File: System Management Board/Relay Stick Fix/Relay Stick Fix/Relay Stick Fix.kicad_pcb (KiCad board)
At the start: 4 copper layers, 28.2 x 27 mm, 17 parts, among them J1 Conn_02x06, Q1 NMOS, U2 74LVC1G04

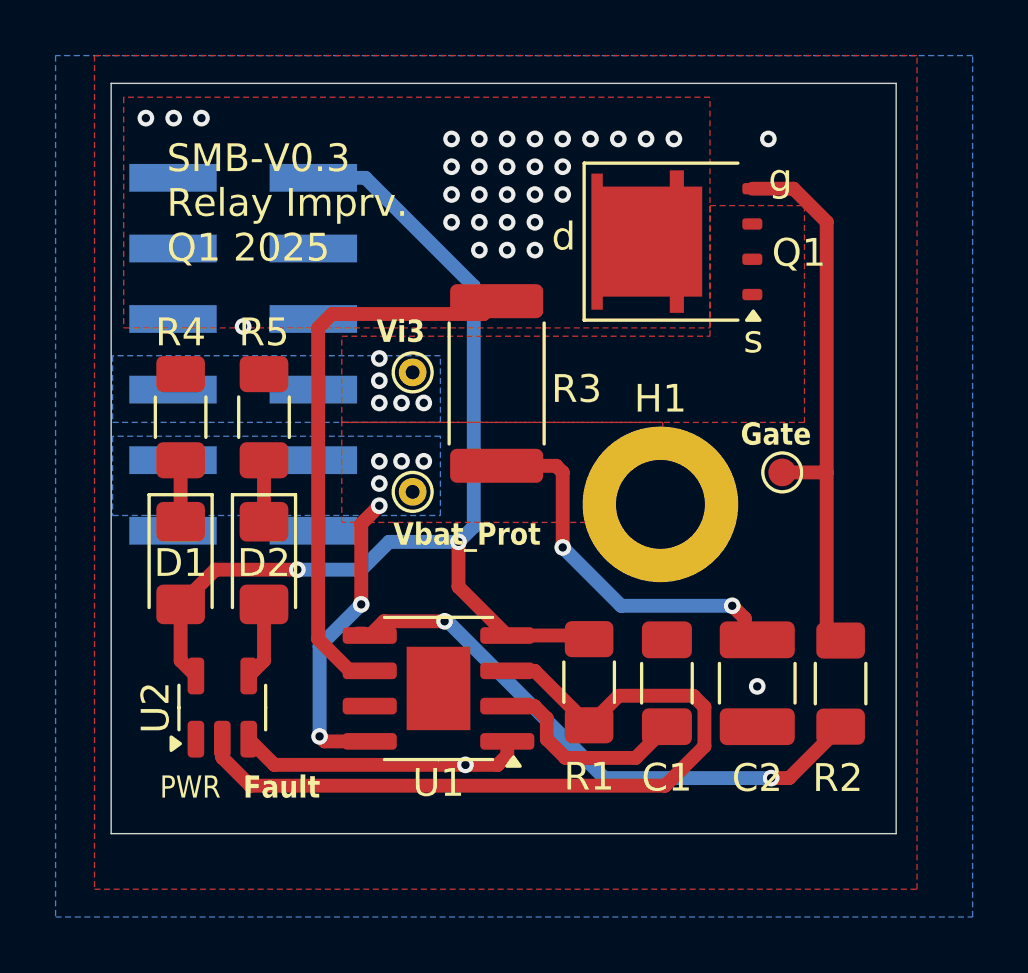
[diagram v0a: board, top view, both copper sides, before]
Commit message: zone fix
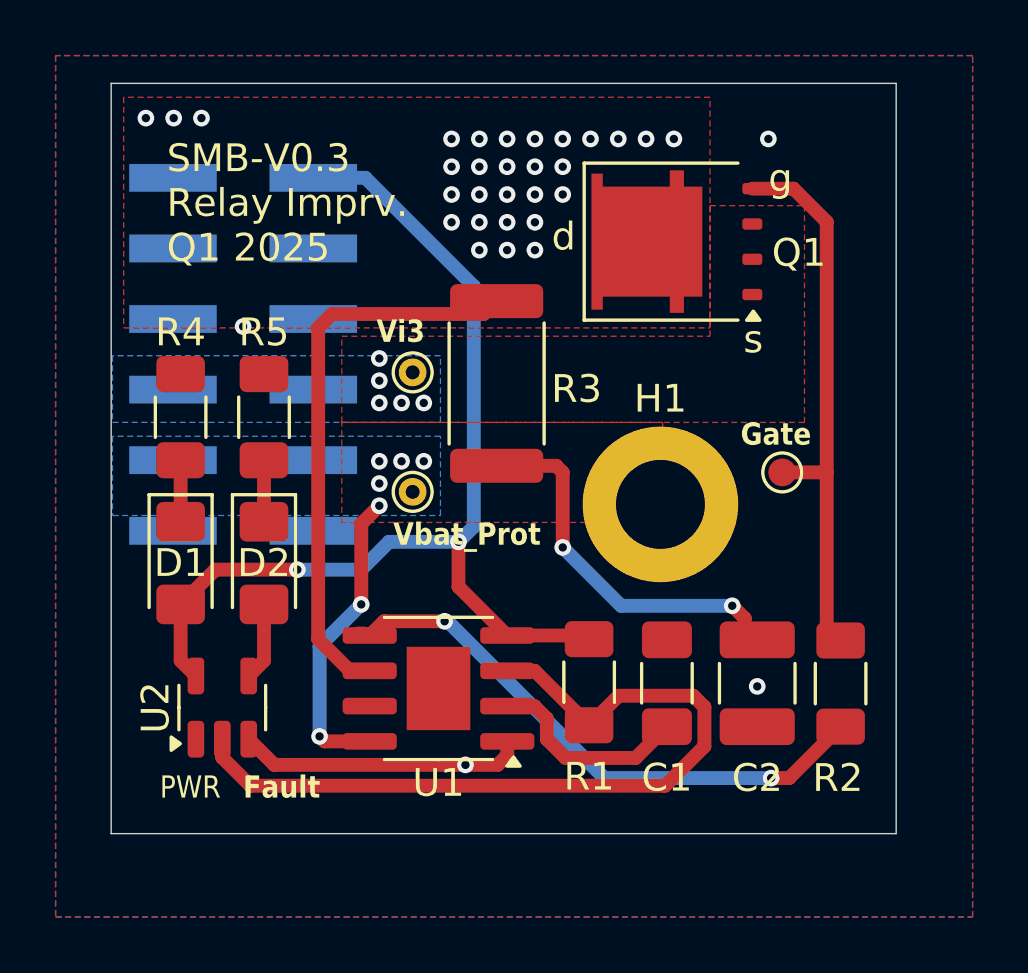
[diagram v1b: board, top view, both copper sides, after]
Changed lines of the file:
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@@
 		(net 1)
 		(net_name "GND")
-		(layers "F.Cu" "In1.Cu")
-		(hatch edge 0.5)
-		(priority 1)
-		(connect_pads
-			(clearance 0.5)
-		)
-		(min_thickness 0.25)
-		(filled_areas_thickness no)
-		(fill yes
-			(thermal_gap 0.5)
-			(thermal_bridge_width 0.5)
-		)
-		(polygon
-			(pts
-				(xy 15.25 14) (xy 15.25 44) (xy 44.85 44) (xy 44.85 14)
-			)
-		)
-	)
-	(zone
-		(net 1)
-		(net_name "GND")
-		(layers "In1.Cu" "B.Cu")
+		(layers "F.Cu" "In1.Cu" "B.Cu")
 		(hatch edge 0.5)
 		(connect_pads
@@
 			)
 		)
+	)
+	(zone
+		(net 6)
+		(net_name "/Sense")
+		(layer "In2.Cu")
+		(hatch edge 0.5)
+		(priority 1)
+		(connect_pads
+			(clearance 0.5)
+		)
+		(min_thickness 0.25)
+		(filled_areas_thickness no)
+		(fill yes
+			(thermal_gap 0.5)
+			(thermal_bridge_width 0.5)
+		)
+		(polygon
+			(pts
+				(xy 15 14.5) (xy 45 14.5) (xy 45 43) (xy 15 43)
+			)
+		)
